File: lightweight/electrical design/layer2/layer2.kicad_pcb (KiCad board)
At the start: 2 copper layers, 208 x 198.4 mm, 50 parts, among them J1 Conn_01x01_Female, J10 Conn_01x01_Female, J11 SH1.0 3P, J14 XH2.54 2P, J15 XT30UPB-F, J16 XT30PW-F, J17 SH1.0 2P, J18 Conn_01x01_Female, J19 Conn_01x01_Female, J2 Conn_01x01_Female, J3 Conn_01x01_Female, J4 Conn_01x01_Female, J5 Conn_01x01_Female, J6 Conn_01x01_Female, J7 Conn_01x01_Female, J8 Conn_01x01_Female, J9 Conn_01x01_Female

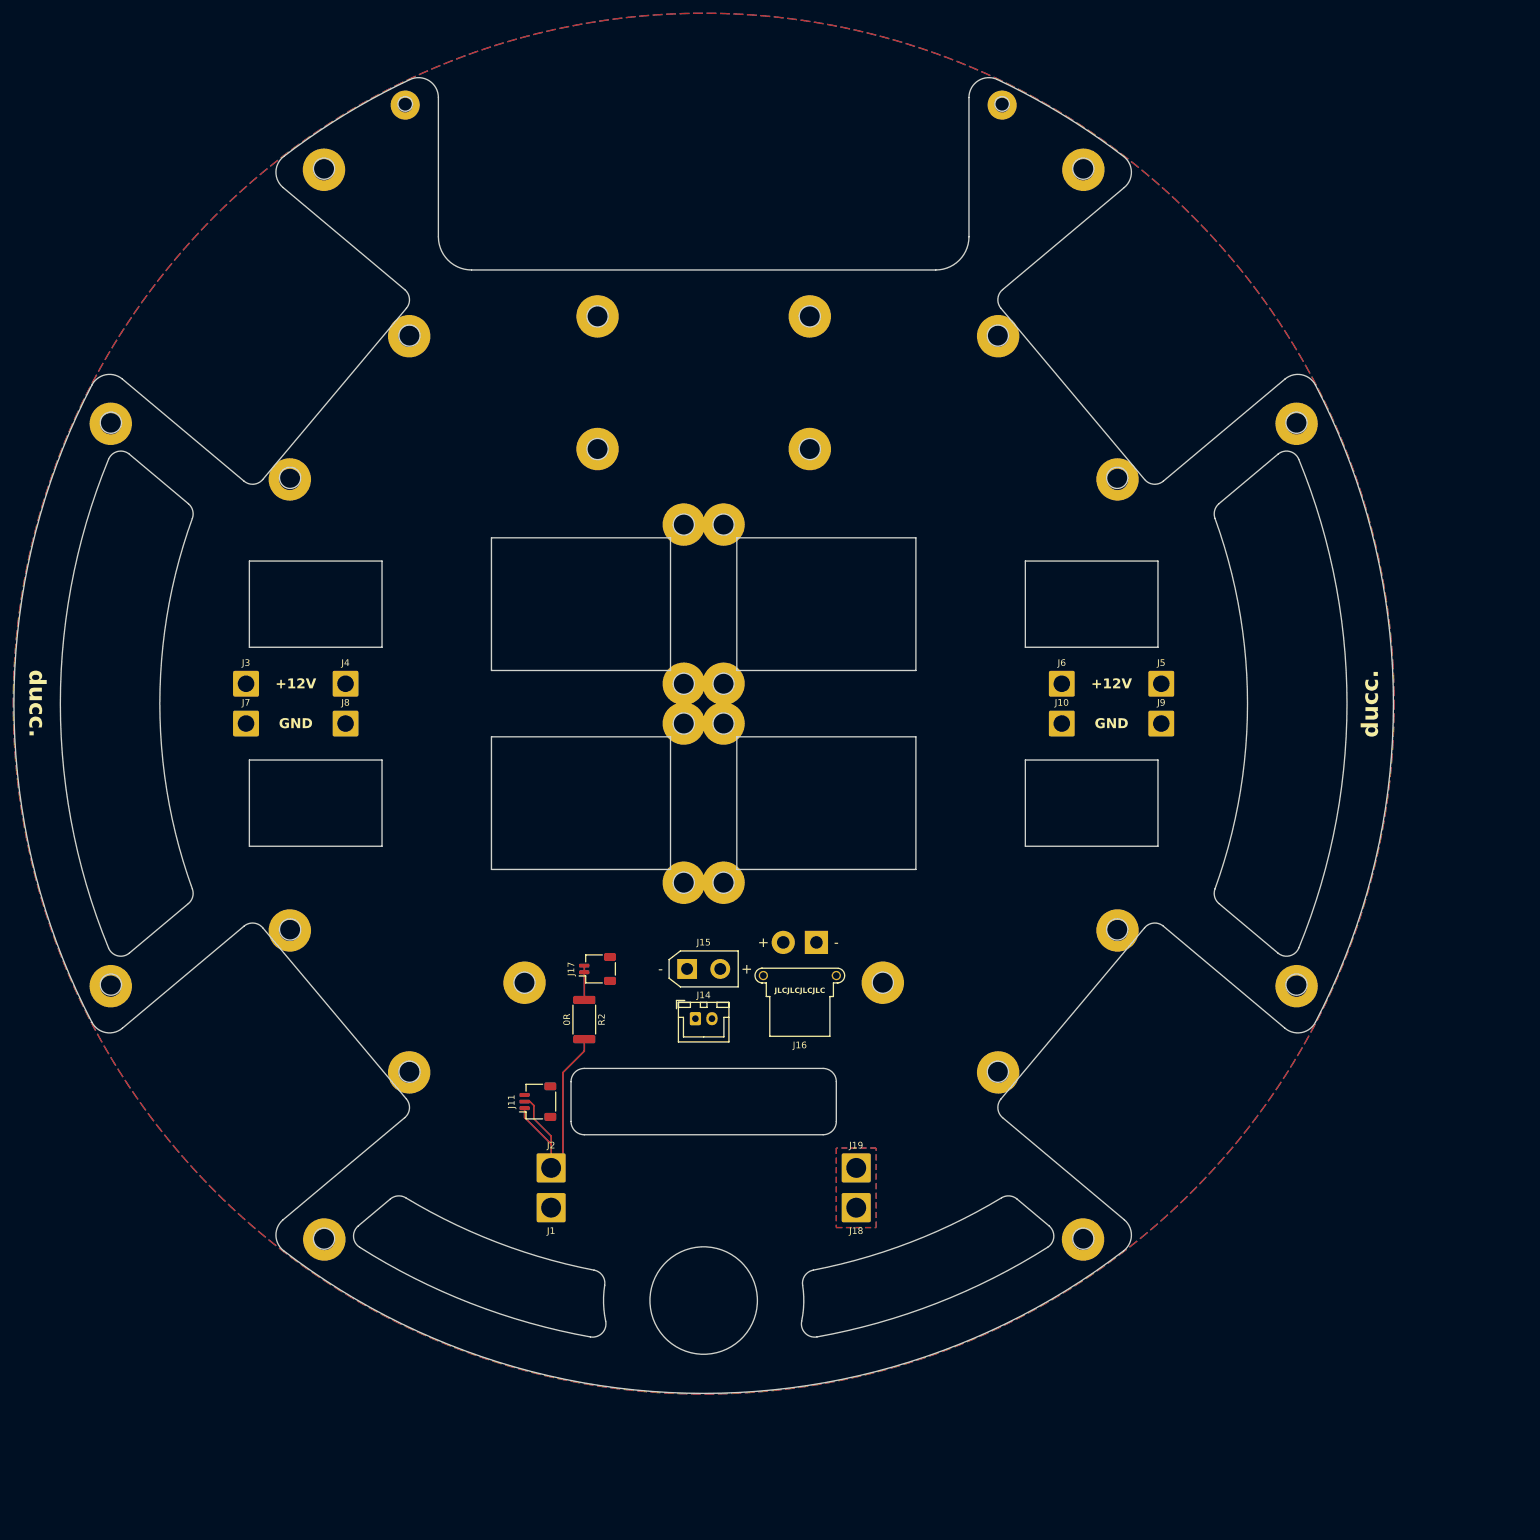
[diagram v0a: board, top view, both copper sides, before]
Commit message: add lw pcb files
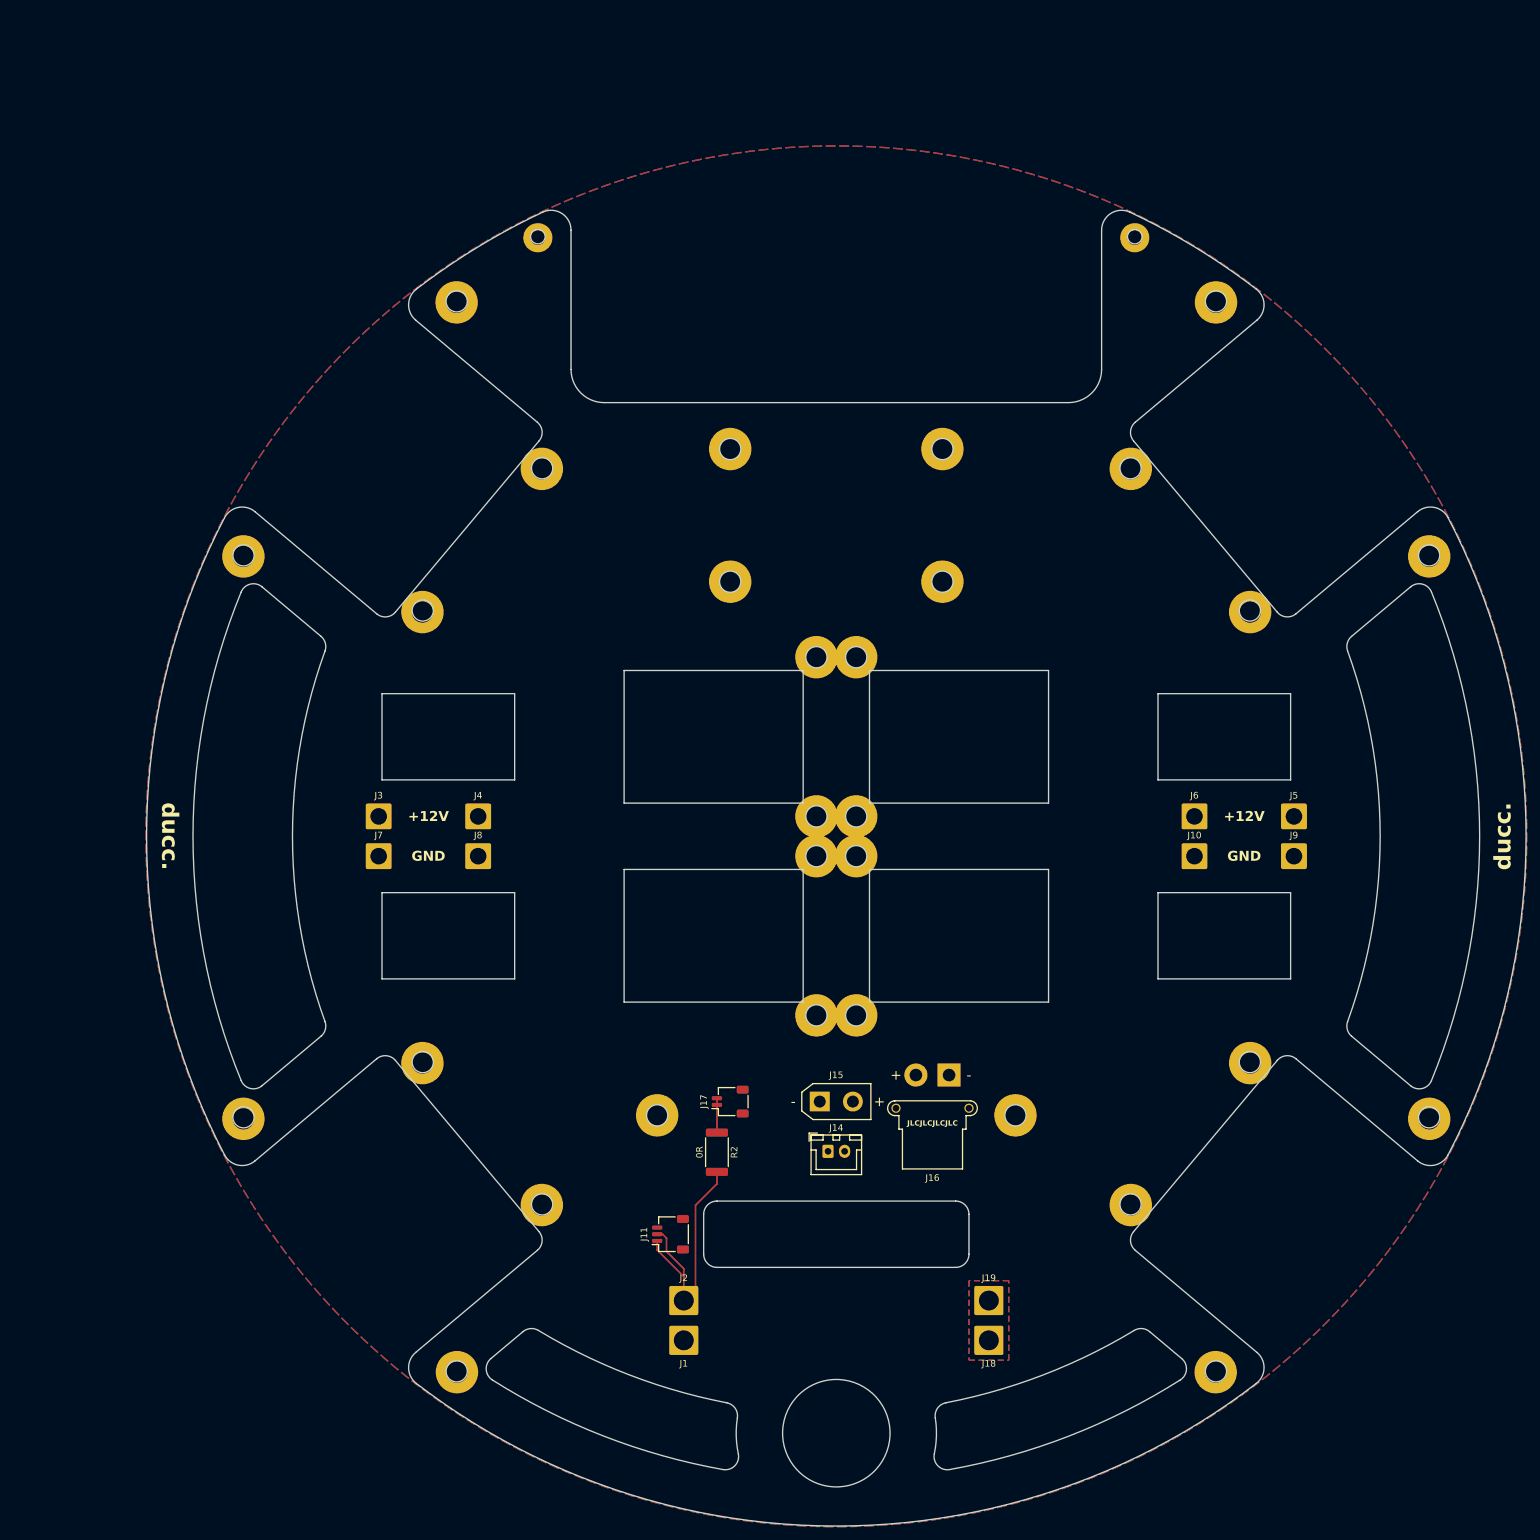
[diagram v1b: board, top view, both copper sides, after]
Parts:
- moved H1 28.3 mm to (67.8, 44.5)
- moved H12 28.3 mm to (187.4, 91.2)
- moved H13 28.3 mm to (187.4, 159.2)
- moved H14 28.3 mm to (169.4, 180.6)
- moved H16 28.3 mm to (62.6, 159.2)
- moved H17 28.3 mm to (122.0, 98.0)
- moved H18 28.3 mm to (122.0, 122.0)
- moved H19 28.3 mm to (128.0, 98.0)
- moved H2 28.3 mm to (182.2, 44.5)
- moved H20 28.3 mm to (128.0, 122.0)
- moved H21 28.3 mm to (128.0, 128.0)
- moved H22 28.3 mm to (128.0, 152.0)
- moved H23 28.3 mm to (122.0, 128.0)
- moved H24 28.3 mm to (122.0, 152.0)
- moved H25 28.3 mm to (98.0, 167.1)
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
